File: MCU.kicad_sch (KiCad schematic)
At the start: 28 parts, among them J1 USB_C_Receptacle_USB2.0_16P, J2 FTSH-105-01-L-DV-K-A, U1 STM32H743VITx, Y1 Crystal_GND24

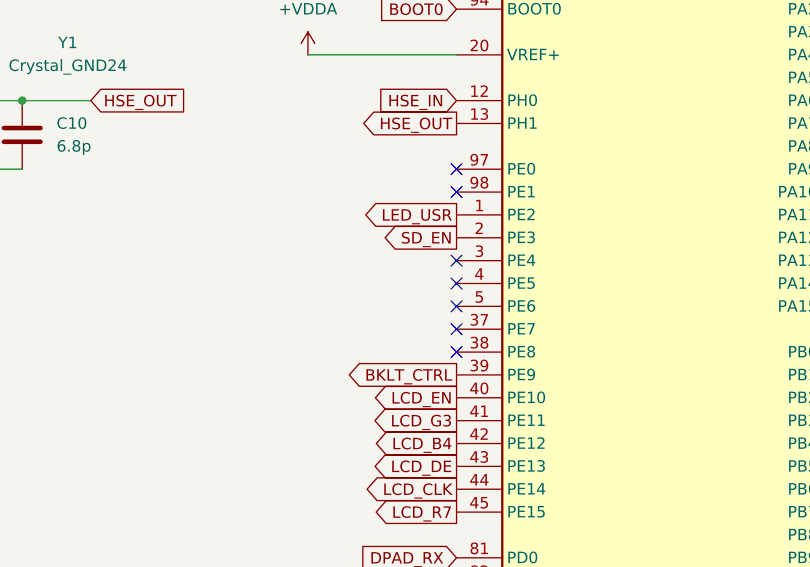
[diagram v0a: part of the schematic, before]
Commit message: r1 final (see changelog.md)
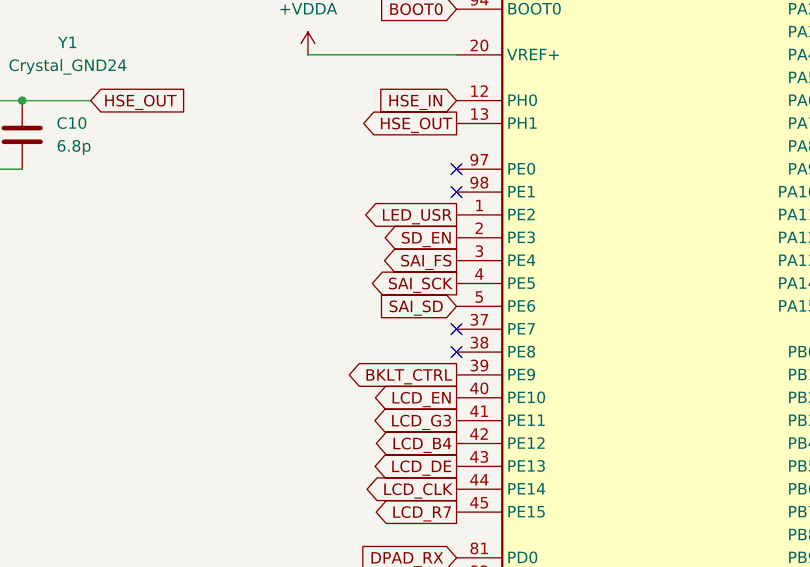
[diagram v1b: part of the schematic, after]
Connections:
- net SAI_FS: now reaches U1.3 (PE4)
- net SAI_SCK: now reaches U1.4 (PE5)
- net SAI_SD: now reaches U1.5 (PE6)
- no-connect marks 26 -> 23
